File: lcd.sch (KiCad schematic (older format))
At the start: 1 part, among them J10 FH26W-33S-0.3SHW

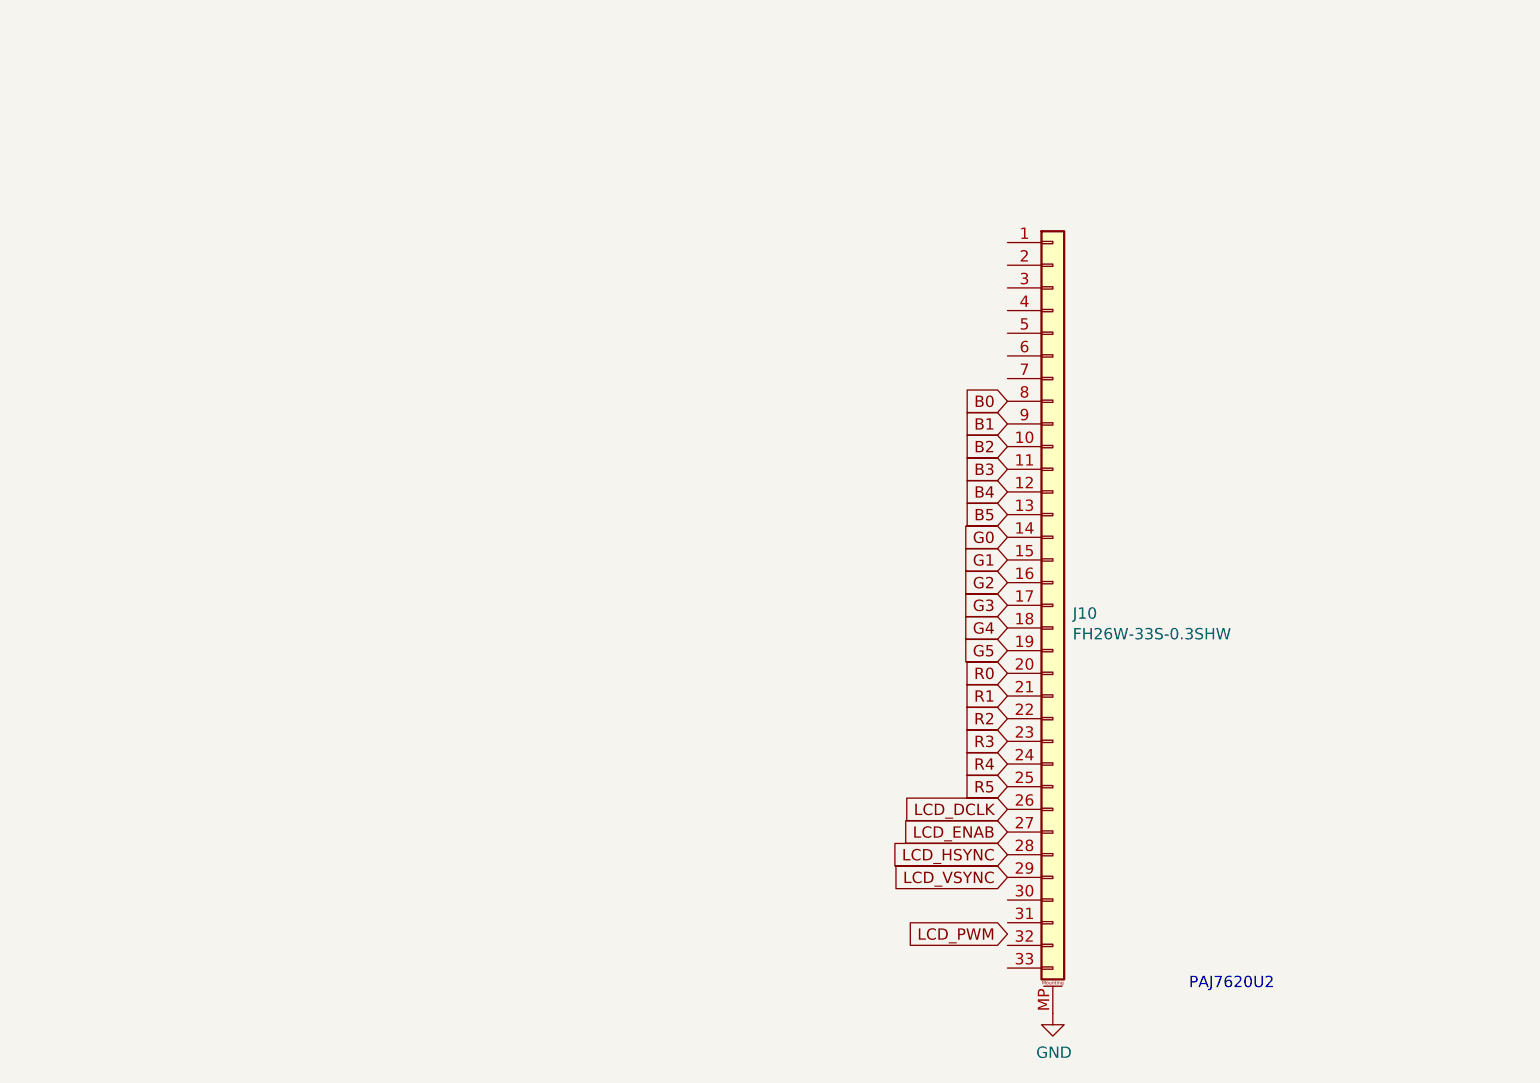
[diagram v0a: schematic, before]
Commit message: layout final?
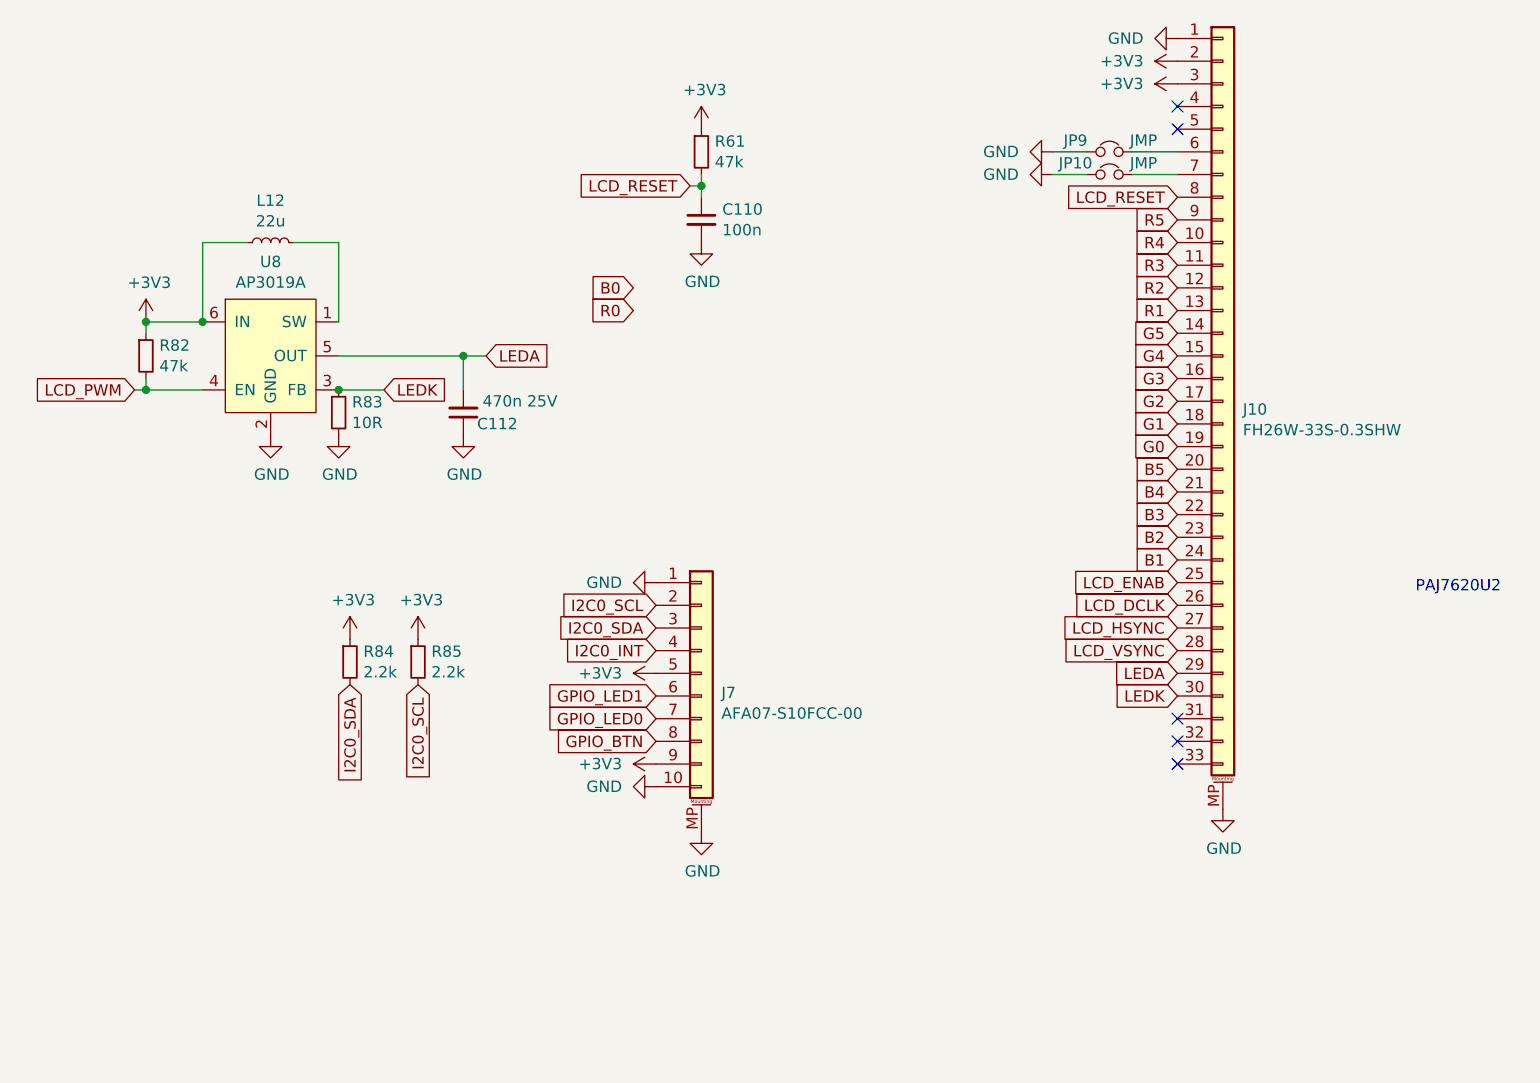
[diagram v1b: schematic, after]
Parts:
- added C110: 100n, otter:C_0402, symbol Device:C_Small
- added C112: 470n 25V, otter:C_0603, symbol Device:C_Small
- added J7: AFA07-S10FCC-00, Connector_FFC-FPC:TE_1-84952-0_1x10-1MP_P1.0mm_Horizontal, symbol Connector_Generic_MountingPin:Conn_01x10_MountingPin
- added JP10, JP9: JMP, Jumper:SolderJumper-2_P1.3mm_Bridged_Pad1.0x1.5mm, symbol Device:Jumper_NC_Small
- added L12: 22u, otter:Inductor_4040, symbol Device:L_Small
- added R61, R82: 47k, otter:R_0402, symbol Device:R_Small
- added R83: 10R, otter:R_0402, symbol Device:R_Small
- added R84, R85: 2.2k, otter:R_0402, symbol Device:R_Small
- added U8: AP3019A, Package_TO_SOT_SMD:SOT-23-6, symbol otter:AP3019A
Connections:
- net B0: no longer J10.8 (Pin_8)
- net B1: now also J10.24 (Pin_24); no longer J10.9 (Pin_9)
- net B2: now also J10.23 (Pin_23); no longer J10.10 (Pin_10)
- net B3: now also J10.22 (Pin_22); no longer J10.11 (Pin_11)
- net B4: now also J10.21 (Pin_21); no longer J10.12 (Pin_12)
- net B5: now also J10.20 (Pin_20); no longer J10.13 (Pin_13)
- net G0: now also J10.19 (Pin_19); no longer J10.14 (Pin_14)
- net G1: now also J10.18 (Pin_18); no longer J10.15 (Pin_15)
- net G2: now also J10.17 (Pin_17); no longer J10.16 (Pin_16)
- net G3: now also J10.16 (Pin_16); no longer J10.17 (Pin_17)
- net G4: now also J10.15 (Pin_15); no longer J10.18 (Pin_18)
- net G5: now also J10.14 (Pin_14); no longer J10.19 (Pin_19)
- net GND: now also J10.1 (Pin_1), C110.2, C112.1, J7.1 (Pin_1), J7.10 (Pin_10), J7.MP (MountPin), JP10.1, JP9.1, R83.2, U8.2 (GND)
- net LCD_ENAB: now also J10.25 (Pin_25); no longer J10.27 (Pin_27)
- net LCD_HSYNC: now also J10.27 (Pin_27); no longer J10.28 (Pin_28)
- net LCD_PWM: now also R82.2, U8.4 (EN)
- net LCD_VSYNC: now also J10.28 (Pin_28); no longer J10.29 (Pin_29)
- net R0: no longer J10.20 (Pin_20)
- net R1: now also J10.13 (Pin_13); no longer J10.21 (Pin_21)
- net R2: now also J10.12 (Pin_12); no longer J10.22 (Pin_22)
- net R3: now also J10.11 (Pin_11); no longer J10.23 (Pin_23)
- net R4: now also J10.10 (Pin_10); no longer J10.24 (Pin_24)
- net R5: now also J10.9 (Pin_9); no longer J10.25 (Pin_25)
- net +3V3: now reaches J10.2 (Pin_2)
- net +3V3: now also J10.3 (Pin_3), J7.5 (Pin_5), J7.9 (Pin_9), L12.1, R61.1, R82.1, R84.1, R85.1, U8.6 (IN)
- net LEDK: now reaches J10.30 (Pin_30)
- net LEDK: now also R83.1, U8.3 (FB)
- net at J10.6 (Pin_6): now also JP9.2
- net at J10.7 (Pin_7): now also JP10.2
- new net: L12.2, U8.1 (SW)
- new net GPIO_BTN: J7.8 (Pin_8)
- new net GPIO_LED0: J7.7 (Pin_7)
- new net GPIO_LED1: J7.6 (Pin_6)
- new net I2C0_INT: J7.4 (Pin_4)
- new net I2C0_SCL: J7.2 (Pin_2), R85.2
- new net I2C0_SDA: J7.3 (Pin_3), R84.2
- new net LCD_RESET: C110.1, J10.8 (Pin_8), R61.2
- new net LEDA: C112.2, J10.29 (Pin_29), U8.5 (OUT)
- no-connect marks 0 -> 5
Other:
- moved on the sheet: J10
